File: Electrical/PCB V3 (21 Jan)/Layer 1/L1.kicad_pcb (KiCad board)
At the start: 2 copper layers, 178 x 170 mm, 197 parts, among them J1 Conn_01x04, U2 CD74HC4067SM, U3 CD74HC4067SM, U5 113991054

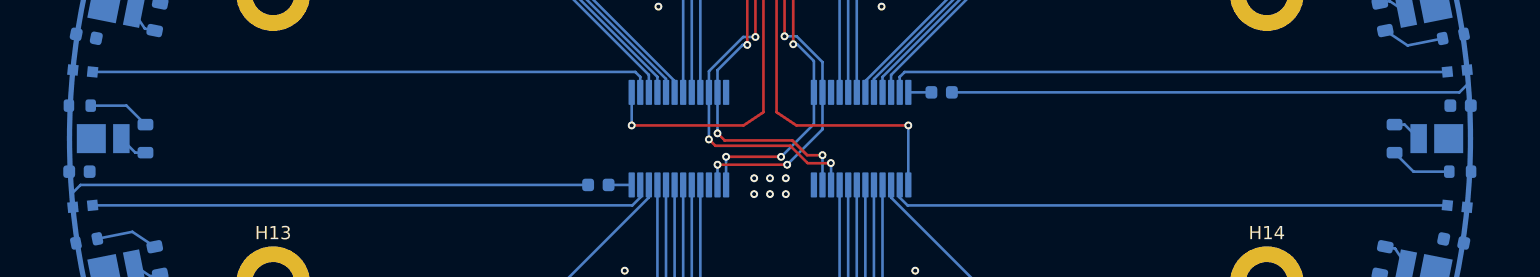
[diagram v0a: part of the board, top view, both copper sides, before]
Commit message: did somemore l1
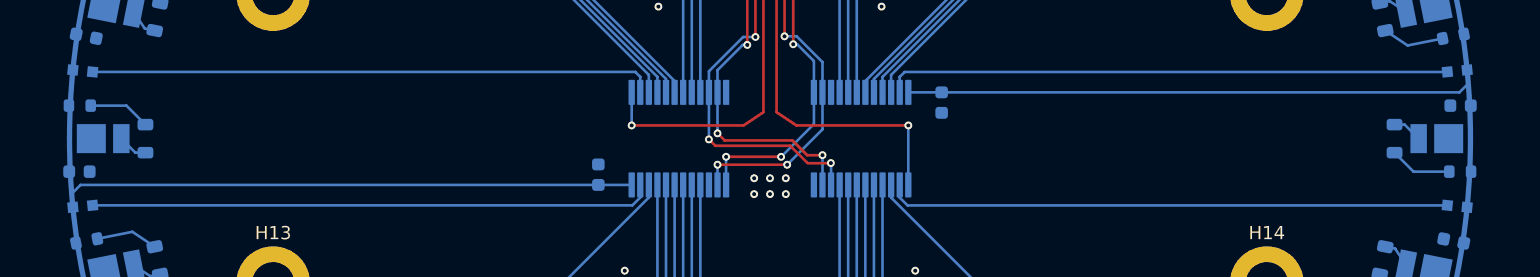
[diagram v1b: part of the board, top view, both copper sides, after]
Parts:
- moved C33 0.78 mm to (100.8, 110.5), turned to -90 degrees
- moved C34 0.78 mm to (126.8, 105.1), turned to 90 degrees
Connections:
- C33 pad 1: +3V3 -> GND
- C33 pad 2: Net-(U3-VCC) -> +3V3
- C34 pad 1: +3V3 -> GND
- C34 pad 2: Net-(U2-VCC) -> +3V3
- U2 pad 24: Net-(U2-VCC) -> +3V3
- U3 pad 24: Net-(U3-VCC) -> +3V3
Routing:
- net +3V3: track 157.3 -> 163.9 mm
- net Net-(U2-VCC): track 1.76 -> 0.00 mm
- net Net-(U3-VCC): track 1.75 -> 0.00 mm
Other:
- board text added: "{dblquote}looks decent lah{dblquote} -yuzhe"
- board text removed: "no"
